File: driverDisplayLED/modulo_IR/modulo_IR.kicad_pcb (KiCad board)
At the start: 2 copper layers, 40 x 18 mm, 16 parts, among them J1 Conn_01x03_Male, U2 LM393

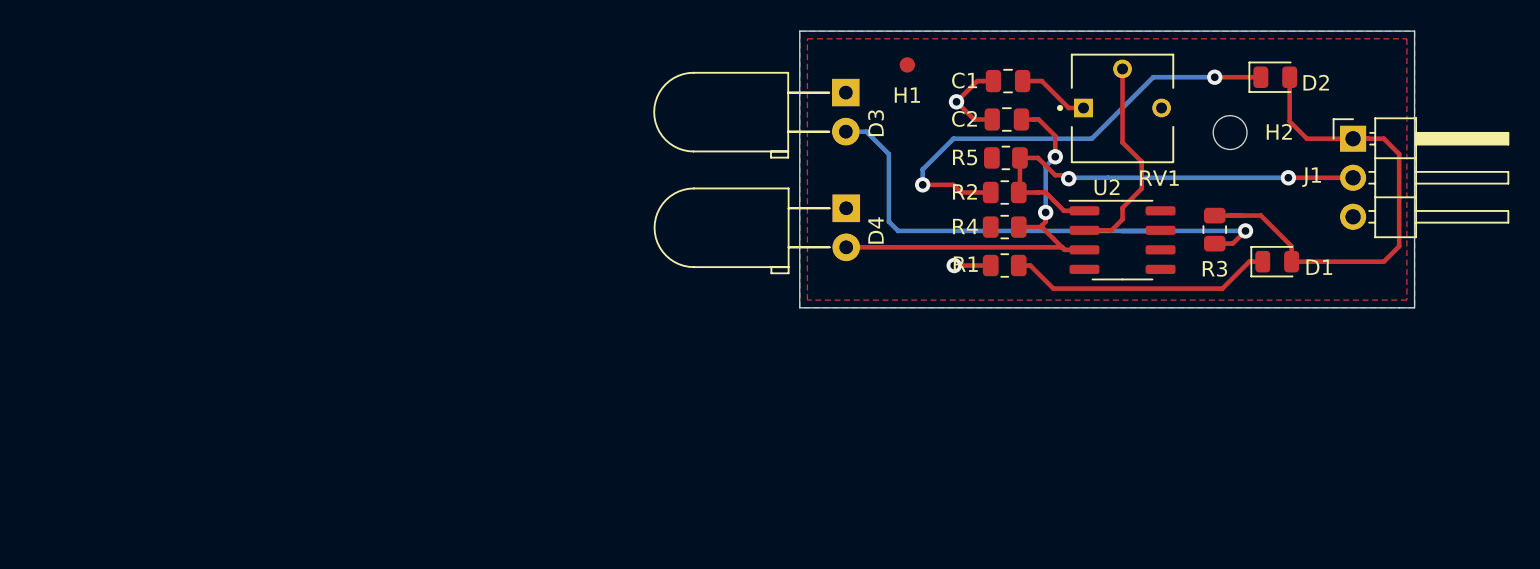
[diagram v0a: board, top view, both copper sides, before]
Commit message: actualizo rotulo
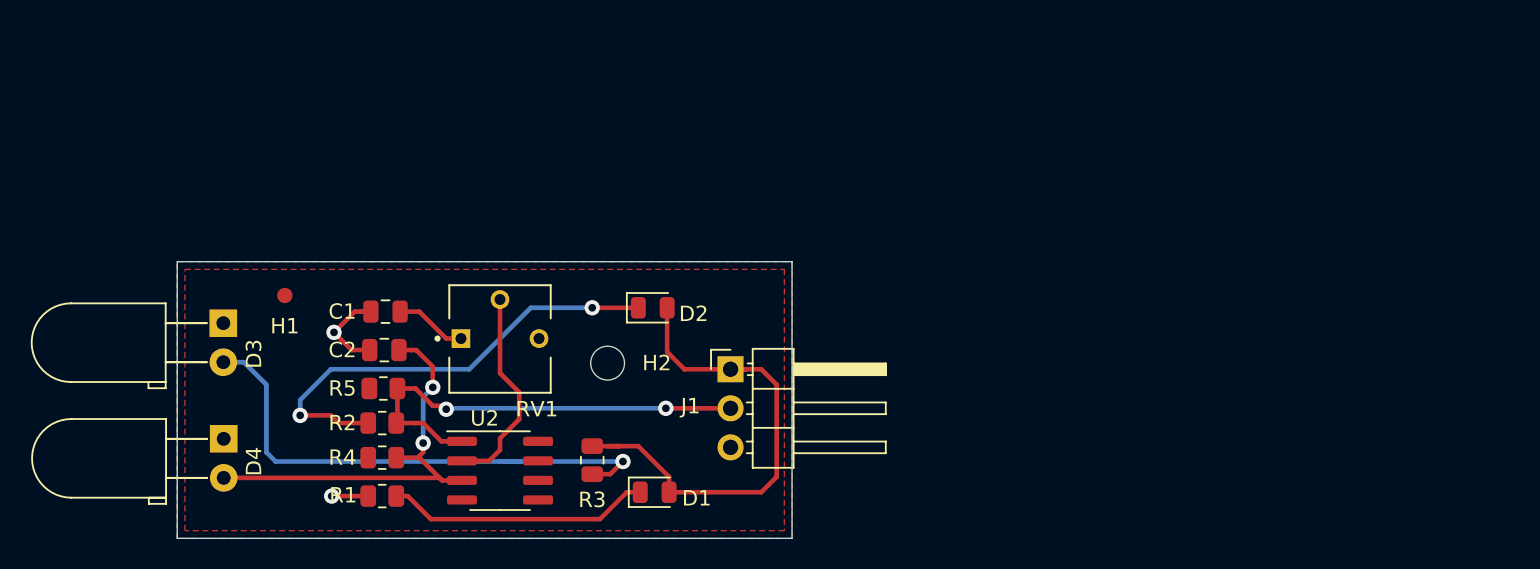
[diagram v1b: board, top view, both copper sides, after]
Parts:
- moved C1 43.2 mm to (81.0, 91.2)
- moved C2 43.2 mm to (81.0, 93.8)
- moved D1 43.2 mm to (98.6, 103.0)
- moved D2 43.2 mm to (98.4, 91.0)
- moved D3 43.2 mm to (70.5, 92.0)
- moved D4 43.2 mm to (70.5, 99.5)
- moved H1 43.2 mm to (74.5, 90.2)
- moved H2 43.2 mm to (95.5, 94.6)
- moved J1 43.2 mm to (103.5, 95.0)
- moved R1 43.2 mm to (80.8, 103.2)
- moved R2 43.2 mm to (80.8, 98.5)
- moved R3 43.2 mm to (94.5, 100.9)
- moved R4 43.2 mm to (80.8, 100.8)
- moved R5 43.2 mm to (80.9, 96.2)
- moved RV1 43.2 mm to (88.5, 93.0)
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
